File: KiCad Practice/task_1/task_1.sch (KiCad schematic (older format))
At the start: 22 parts, among them Q1 2N3904, SW1 SW_Push, U1 MIC5219-2.8YM5, U2 STM8L051F3P

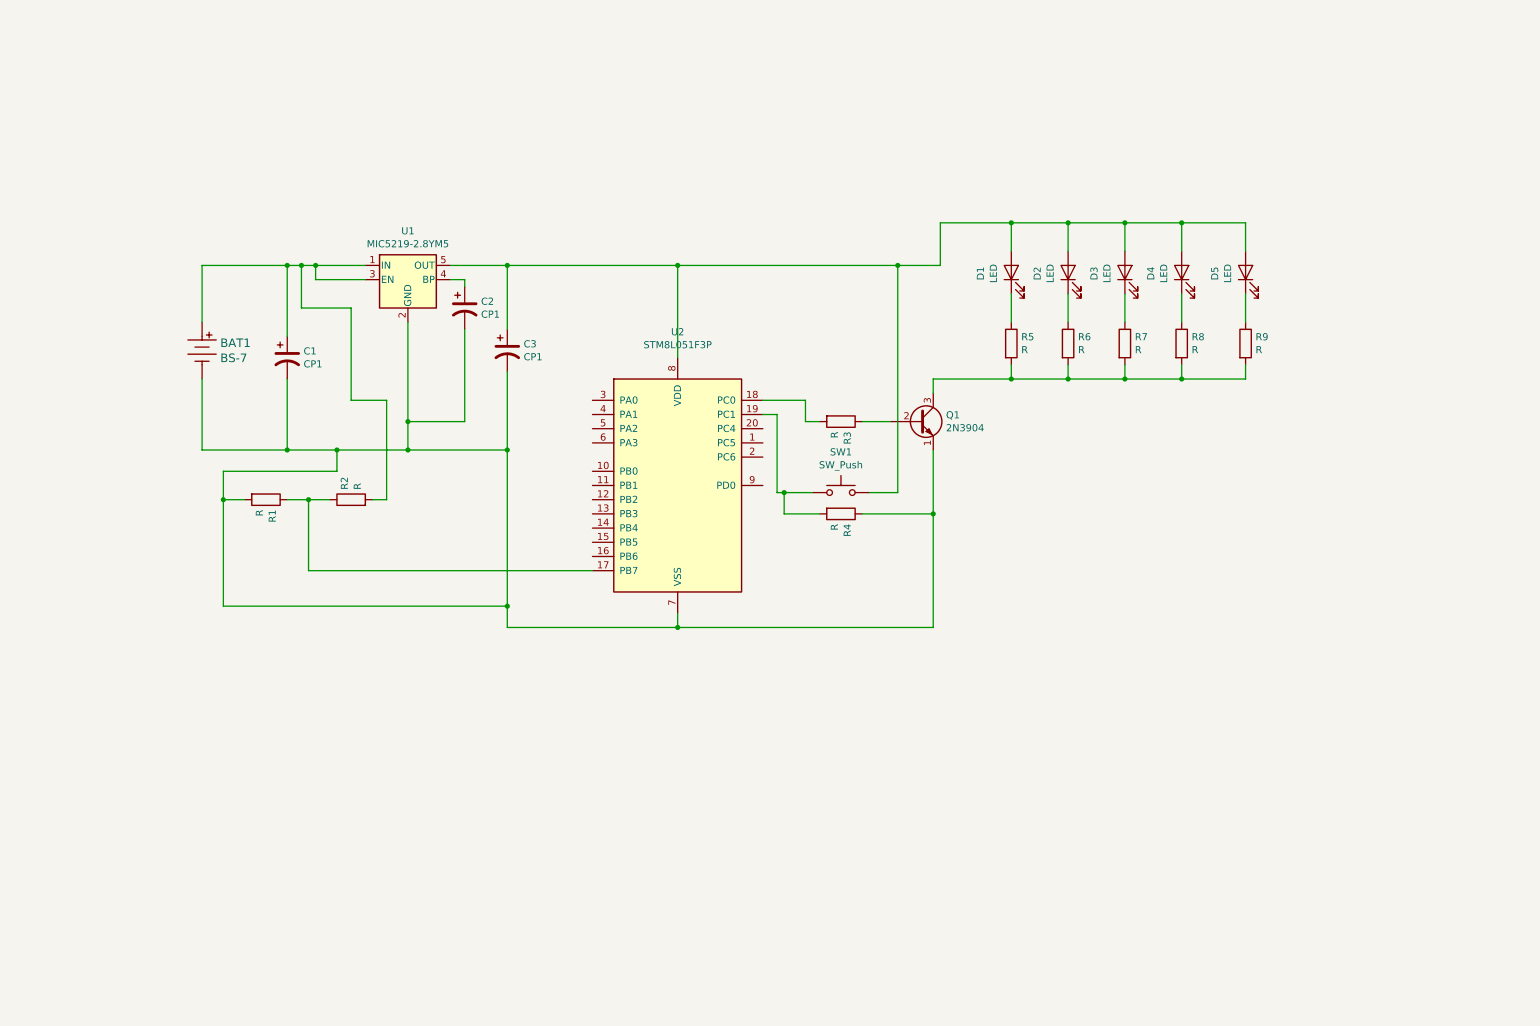
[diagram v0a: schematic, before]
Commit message: made schematic
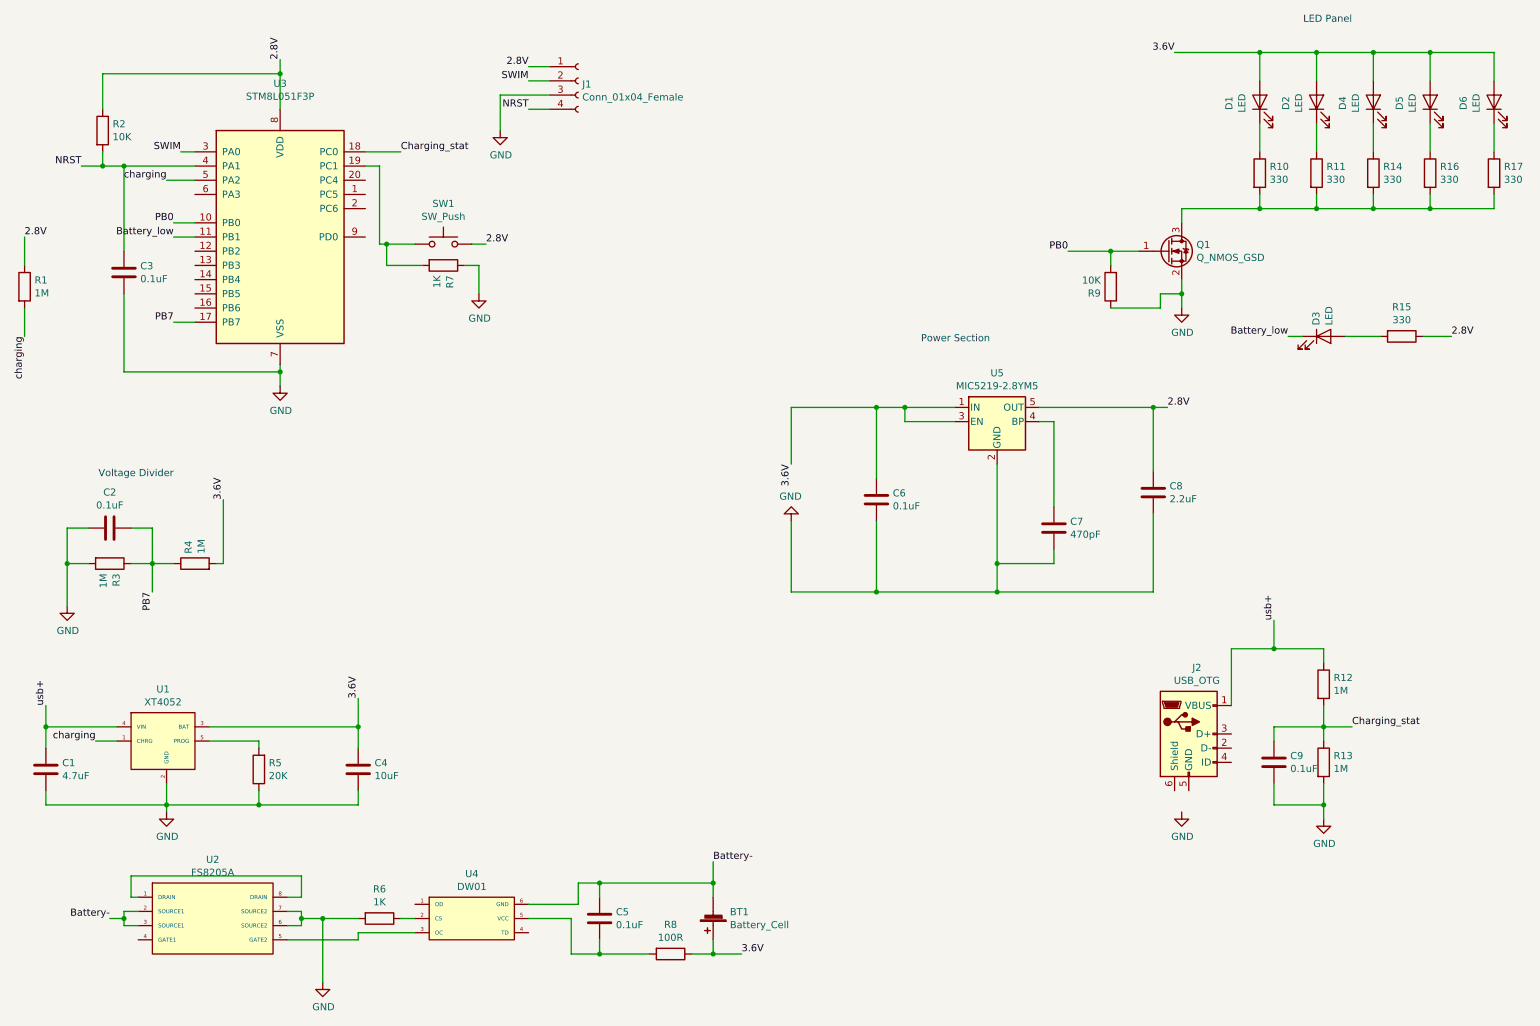
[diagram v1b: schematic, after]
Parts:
- removed BAT1: BS-7, digikey-footprints:Battery_Holder_Coin_2032_BS-7, symbol dk_Battery-Holders-Clips-Contacts:BS-7
- removed C1, C2, C3: CP1, symbol Device:CP1
- removed Q1: 2N3904, Package_TO_SOT_THT:TO-92_Inline, symbol Transistor_BJT:2N3904
- added BT1: Battery_Cell, symbol Device:Battery_Cell
- added C1: 4.7uF, Capacitor_SMD:C_0603_1608Metric, symbol Device:C
- added C2, C3, C5, C6, C9: 0.1uF, Capacitor_SMD:C_0603_1608Metric, symbol Device:C
- added C4: 10uF, Capacitor_SMD:C_0603_1608Metric, symbol Device:C
- added C7: 470pF, Capacitor_SMD:C_0603_1608Metric, symbol Device:C
- added C8: 2.2uF, Capacitor_SMD:C_0603_1608Metric, symbol Device:C
- added D3: LED, LED_SMD:LED_0805_2012Metric, symbol Device:LED
- added J1: Conn_01x04_Female, symbol Connector:Conn_01x04_Female
- added J2: USB_OTG, symbol Connector:USB_OTG
- added Q1: Q_NMOS_GSD, symbol Device:Q_NMOS_GSD
- added R1, R12, R13: 1M, Capacitor_SMD:C_0201_0603Metric, symbol Device:R
- added R15: 330, Capacitor_SMD:C_0201_0603Metric, symbol Device:R
- added R2: 10K, Capacitor_SMD:C_0201_0603Metric, symbol Device:R
- added R5: 20K, Capacitor_SMD:C_0201_0603Metric, symbol Device:R
- added R6: 1K, Capacitor_SMD:C_0201_0603Metric, symbol Device:R
- added R8: 100R, Capacitor_SMD:C_0201_0603Metric, symbol Device:R
- added U1: XT4052, symbol comps:XT4052
- added U2: FS8205A, symbol comps:FS8205A
- added U4: DW01, symbol comps:DW01
- D1, D2: footprint (none) -> LED_SMD:LED_0805_2012Metric
- D4: renamed from D3; footprint (none) -> LED_SMD:LED_0805_2012Metric
- D5: renamed from D4; footprint (none) -> LED_SMD:LED_0805_2012Metric
- D6: renamed from D5; footprint (none) -> LED_SMD:LED_0805_2012Metric
- R10: renamed from R5; value R -> 330; footprint (none) -> Capacitor_SMD:C_0201_0603Metric
- R11: renamed from R6; value R -> 330; footprint (none) -> Capacitor_SMD:C_0201_0603Metric
- R14: renamed from R7; value R -> 330; footprint (none) -> Capacitor_SMD:C_0201_0603Metric
- R16: renamed from R8; value R -> 330; footprint (none) -> Capacitor_SMD:C_0201_0603Metric
- R17: renamed from R9; value R -> 330; footprint (none) -> Capacitor_SMD:C_0201_0603Metric
- R3: renamed from R1; value R -> 1M; footprint (none) -> Capacitor_SMD:C_0201_0603Metric
- R4: renamed from R2; value R -> 1M; footprint (none) -> Capacitor_SMD:C_0201_0603Metric
- R7: renamed from R4; value R -> 1K; footprint (none) -> Capacitor_SMD:C_0201_0603Metric
- R9: renamed from R3; value R -> 10K; footprint (none) -> Capacitor_SMD:C_0201_0603Metric
- renumbered U2 to U3, U1 to U5
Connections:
- net PB0: now reaches U3.10 (PB0)
- net PB0: now also R9.2, Q1.1 (G)
- net Battery_low: now reaches U3.11 (PB1)
- net Battery_low: now also D3.1 (K)
- net PB7: now reaches R3.1, R4.1, U3.17 (PB7)
- net PB7: now also C2.2
- net Charging_stat: now reaches U3.18 (PC0)
- net Charging_stat: now also C9.1, R12.2, R13.1; no longer R9.2
- net SWIM: now reaches U3.3 (PA0)
- net SWIM: now also J1.2 (Pin_2)
- net NRST: now reaches U3.4 (PA1)
- net NRST: now also C3.1, J1.4 (Pin_4), R2.2
- net charging: now reaches U3.5 (PA2)
- net charging: now also R1.2, U1.1 (CHRG)
- net GND: now reaches R3.2, R7.1, U3.7 (VSS), U5.2 (GND)
- net GND: now also R9.1, C1.2, C2.1, C3.2, C4.2, C6.2, C7.2, C8.2, C9.2, J1.3 (Pin_3), Q1.2 (S), R13.2, R5.1, R6.2, U1.2 (GND), U2.6 (SOURCE2), U2.7 (SOURCE2)
- net 3.6V: now reaches D1.2 (A), D2.2 (A), D4.2 (A), D5.2 (A), D6.2 (A)
- net 3.6V: now also R4.2, U5.1 (IN), U5.3 (EN), BT1.1 (+), C4.1, C6.1, R8.1, U1.3 (BAT); no longer SW1.2, U3.8 (VDD), U5.5 (OUT)
- net at U5.4 (BP): now also C7.1
- net at R10.2, R11.2, R14.2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: now also Q1.3 (D)
- new net: U2.1 (DRAIN), U2.8 (DRAIN)
- new net: U2.5 (GATE2), U4.3 (OC)
- new net: R6.1, U4.2 (CS)
- new net: C5.2, R8.2, U4.5 (VCC)
- new net: D3.2 (A), R15.2
- new net: R5.2, U1.5 (PROG)
- new net 2.8V: C8.1, J1.1 (Pin_1), R1.1, R15.1, R2.1, SW1.2, U3.8 (VDD), U5.5 (OUT)
- new net Battery-: BT1.2 (-), C5.1, U2.2 (SOURCE1), U2.3 (SOURCE1), U4.6 (GND)
- new net usb+: C1.1, J2.1 (VBUS), R12.1, U1.4 (VIN)
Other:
- note added: "LED Panel"
- note added: "Power Section"
- note added: "Voltage Divider\n"
- moved on the sheet: D1, D2, D4, D5, D6, R10, R11, R14, R16, R17, R3, R4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
